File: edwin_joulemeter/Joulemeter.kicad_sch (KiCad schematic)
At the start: 17 parts, among them J1 Conn_01x02, J2 Conn_01x02, U1 INA240A3PWR, U2 ADS131M04IRUKR, U3 TLV709A01DBVR, U4 TPS7B92050DBVR

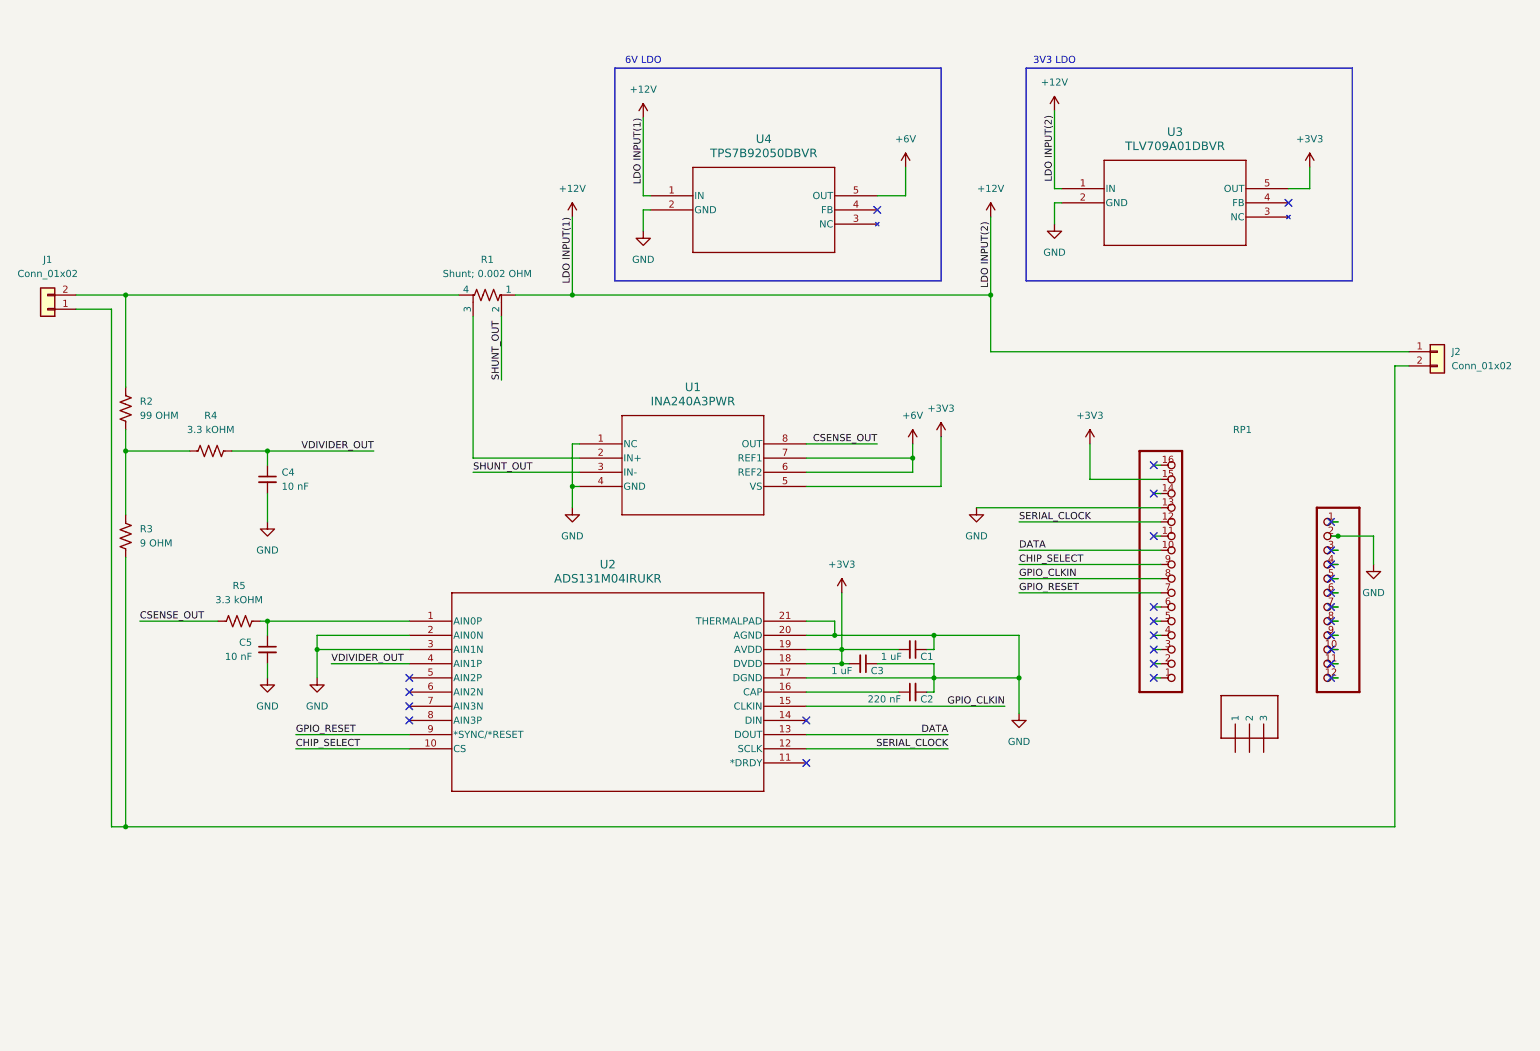
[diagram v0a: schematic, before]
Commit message: updated 1/5/25
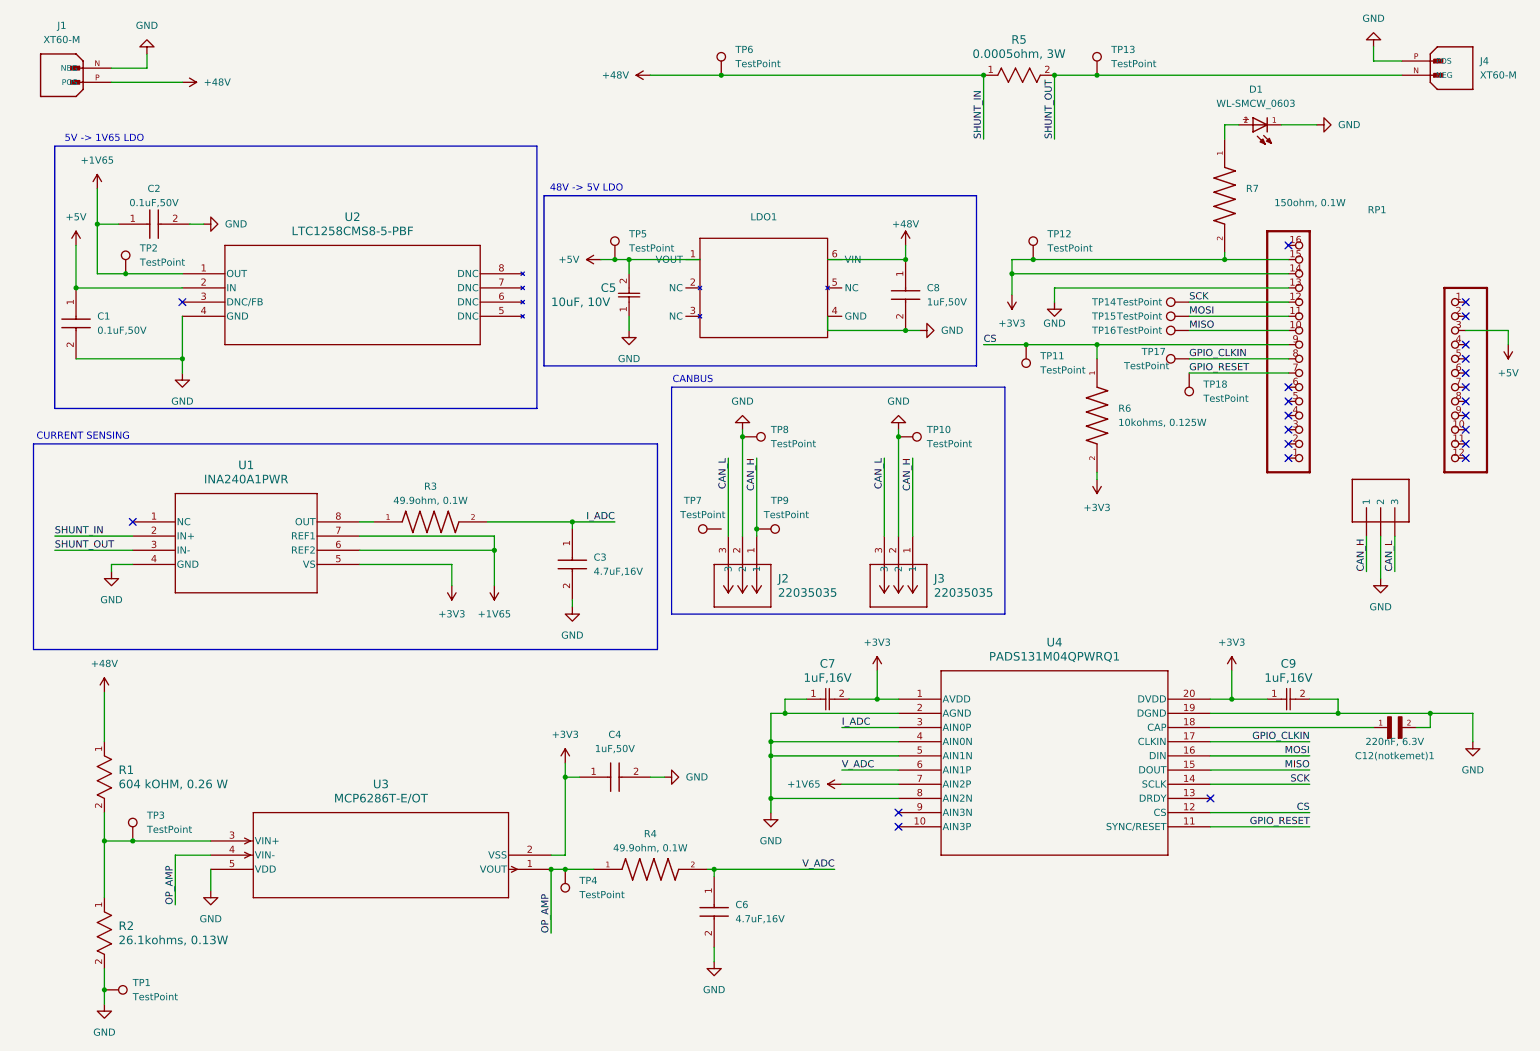
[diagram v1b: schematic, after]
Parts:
- removed C1, C3: 1 uF, symbol Device:C_Small
- removed C2: 220 nF, symbol Device:C_Small
- removed C4, C5: 10 nF, symbol Device:C_Small
- removed J1, J2: Conn_01x02, symbol Connector_Generic:Conn_01x02
- removed R1: Shunt; 0.002 OHM, symbol Device:R_Shunt_US
- removed R2: 99 OHM, symbol Device:R_US
- removed R3: 9 OHM, symbol Device:R_US
- removed R4, R5: 3.3 kOHM, symbol Device:R_US
- removed U2: ADS131M04IRUKR, RUK20_TEX, symbol Joulemeter:ADS131M04IRUKR
- removed U3: TLV709A01DBVR, SOT-23-5_DBV_TEX, symbol Joulemeter:TLV709A01DBVR
- removed U4: TPS7B92050DBVR, SOT-23-5_DBV_TEX, symbol Joulemeter:TLV709A01DBVR
- added C1, C2: 0.1uF,50V, C0805, symbol SMV_Custom:C0805C104K5RACTU
- added C12(notkemet)1: 220nF, 6.3V, SMV_Passives:0805RESC2012X60N, symbol SMV_Custom:GCM188R71H104KA57D
- added C3, C6: 4.7uF,16V, SMV_Passives:Cap0805, symbol SMV_Custom:C0805C475K4RACTU
- added C4, C8: 1uF,50V, C0805, symbol SMV_Custom:C0805C102K5GACTU
- added C5: 10uF, 10V, CAP_8PACTU, symbol SMV_Custom:C0805C106K8PACTU
- added C7, C9: 1uF,16V, SMV_Passives:Cap0805, symbol SMV_Custom:C0805C105K4RACTU
- added D1: WL-SMCW_0603, WL-SMCW_0603:WL-SMCW_0603, symbol SMV_Custom:WL-SMCW_0603
- added J1, J4: XT60-M, XT60-M:AMASS_XT60-M, symbol SMV_Custom:XT60-M
- added J2, J3: 22035035, CON_22035035_MOL, symbol SMV_Custom:3-pin Mini Molex Spox
- added LDO1: ~, symbol SMV_Custom:AP7387-50FDCR-7
- added R1: 604 kOHM, 0.26 W, RES_TNPW0805_VIS, symbol SMV_Custom:TNPW0805604KBEEA
- added R2: 26.1kohms, 0.13W, RES_TNPW0402_VIS, symbol SMV_Custom:TNPW040226K1BEED
- added R3, R4: 49.9ohm, 0.1W, CRCW060349R9FKEAC:RESC1608X55N, symbol SMV_Custom:CRCW060349R9FKEAC
- added R5: 0.0005ohm, 3W, RES_PU3921_.5mOHM_YAG, symbol SMV_Custom:PU3921FKM130U5L
- added R6: 10kohms, 0.125W, CRCW080510K0FKEAC:RESC2012X60N, symbol SMV_Custom:CRCW080510K0FKEAC
- added R7: 150ohm, 0.1W, CRCW0603150RFKEAC:RESC1608X55N, symbol SMV_Custom:CRCW0603150RFKEAC
- added TP1, TP10, TP11, TP12, TP13, TP14, TP15, TP16, TP17, TP18, TP2, TP3, TP4, TP5, TP6, TP7, TP8, TP9: TestPoint, TestPoint:TestPoint_Pad_3.0x3.0mm, symbol Connector:TestPoint
- added U2: LTC1258CMS8-5-PBF, MSOP-8_MS_LIT, symbol SMV_Custom:LTC1258CMS8-5-PBF
- added U3: MCP6286T-E/OT, SOT-23-5_MC_MCH, symbol SMV_Custom:MCP6286T-E_OT
- added U4: PADS131M04QPWRQ1, SMV_ICs:TSSOP20_PW_TEX, symbol SMV_Custom:PADS131M04QPWRQ1
- U1: value INA240A3PWR -> INA240A1PWR
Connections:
- net CHIP_SELECT is gone; now on net CS: RP1.9
- net DATA is gone; now on net MISO: RP1.10
- net SERIAL_CLOCK is gone; now on net SCK: RP1.12
- net +3V3: now also RP1.14, C4.1, C7.2, C9.1, R6.2, R7.2, TP12.1, U3.2 (VSS), U4.1 (AVDD), U4.20 (DVDD)
- net GND: now also C1.2, C12(notkemet)1.2, C2.2, C3.2, C4.2, C5.1, C6.2, C7.1, C8.2, C9.2, D1.1, J1.N (NEG), J2.2, J3.2, J4.P (POS), LDO1.4 (GND), R2.2, TP1.1, TP10.1, TP8.1, U2.4 (GND), U3.5 (VDD), U4.19 (DGND), U4.2 (AGND), U4.4 (AIN0N), U4.5 (AIN1N), U4.8 (AIN2N); no longer U1.1 (NC)
- net GPIO_CLKIN: now also TP17.1, U4.17 (CLKIN)
- net GPIO_RESET: now also TP18.1, U4.11 (SYNC/RESET)
- net SHUNT_OUT: now also J4.N (NEG), R5.2, TP13.1
- net +48V: now reaches U1.2 (IN+)
- net +48V: now also C8.1, J1.P (POS), LDO1.6 (VIN), R1.1, R5.1, TP6.1
- net CAN_H: now reaches RP1.1
- net CAN_H: now also J2.1, J3.1, TP9.1
- net MISO: now reaches RP1.10
- net MISO: now also TP16.1, U4.15 (DOUT)
- net MOSI: now reaches RP1.11
- net MOSI: now also TP15.1, U4.16 (DIN)
- net SCK: now reaches RP1.12
- net SCK: now also TP14.1, U4.14 (SCLK)
- net CAN_L: now reaches RP1.3
- net CAN_L: now also J2.3, J3.3
- net CS: now reaches RP1.9
- net CS: now also R6.1, TP11.1, U4.12 (CS)
- net +6V renamed +1V65
- net +1V65: now also C2.1, TP2.1, U2.1 (OUT), U4.7 (AIN2P)
- net CSENSE_OUT: no longer names the net of U1.8 (OUT)
- net CSENSE_OUT: now also R3.1
- new net: R1.2, R2.1, TP3.1, U3.3 (VIN+)
- new net: C12(notkemet)1.1, U4.18 (CAP)
- new net: D1.2, R7.1
- new net +5V: C1.1, C5.2, LDO1.1 (VOUT), RP1.3, TP5.1, U2.2 (IN)
- new net I_ADC: C3.1, R3.2, U4.3 (AIN0P)
- new net OP_AMP: R4.1, TP4.1, U3.1 (VOUT), U3.4 (VIN-)
- new net V_ADC: C6.1, R4.2, U4.6 (AIN1P)
- no-connect marks 28 -> 23
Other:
- note added: "48V -> 5V LDO"
- note added: "5V -> 1V65 LDO"
- note added: "CANBUS"
- note added: "CURRENT SENSING"
- note removed: "3V3 LDO"
- note removed: "6V LDO"

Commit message: updates to pcb/schematic for 1/7/2025
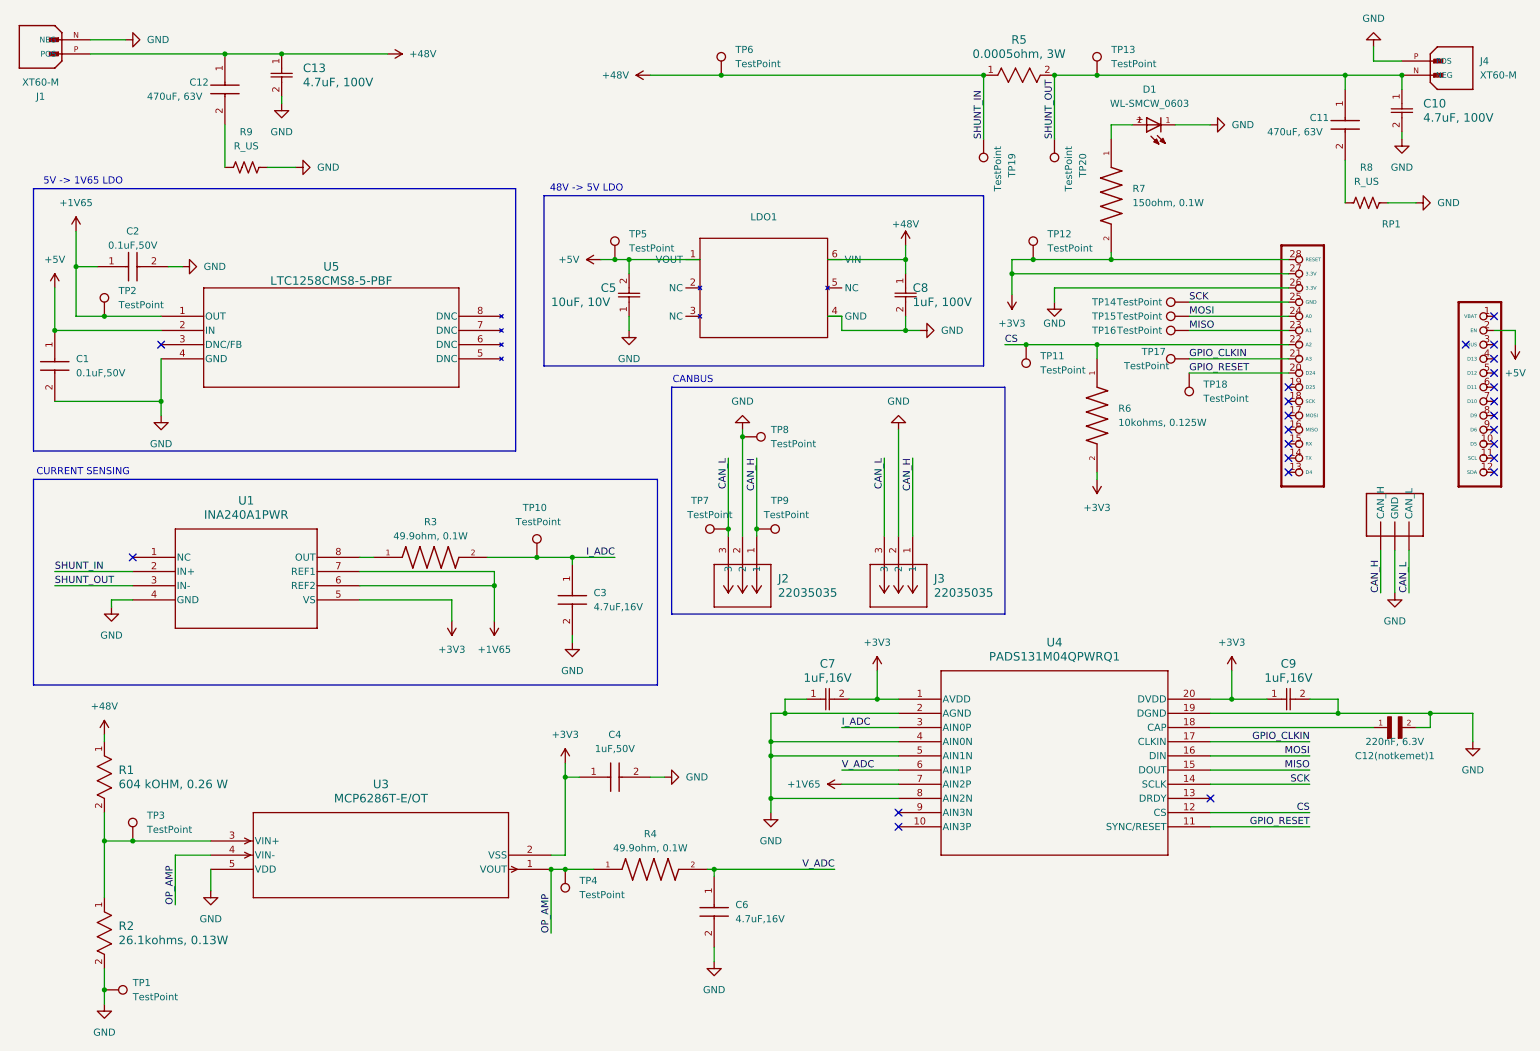
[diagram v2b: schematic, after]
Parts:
- removed C8: 1uF,50V, C0805, symbol SMV_Custom:C0805C102K5GACTU
- removed U2: LTC1258CMS8-5-PBF, MSOP-8_MS_LIT, symbol SMV_Custom:LTC1258CMS8-5-PBF
- added C10: 4.7uF, 100V, SMV_Passives:CAP_C2220C_2S_KEM, symbol SMV_Custom:C2220C475M1R2C7186
- added C11, C12: 470uF, 63V, SMV_Passives:Big_Chunky_Cap, symbol SMV_Custom:Big_Chunky_Cap2
- added C13: 4.7uF, 100V, CAP_C2220C_2S_KEM, symbol SMV_Custom:C2220C475M1R2C7186
- added C8: 1uF, 100V, SMV_Passives:CAPC340180_180N_KEM, symbol SMV_Custom:C1206C105K1RACTU
- added R8, R9: R_US, Resistor_THT:R_Axial_DIN0204_L3.6mm_D1.6mm_P1.90mm_Vertical, symbol Device:R_US
- added TP19, TP20: TestPoint, TestPoint:TestPoint_Pad_3.0x3.0mm, symbol Connector:TestPoint
- added U5: LTC1258CMS8-5-PBF, SMV_ICs:MSOP-8_MS_LIT, symbol SMV_Custom:LTC1258CMS8-5-PBF
- C1, C2, C4: footprint C0805 -> SMV_Passives:Cap0805
- C5: footprint CAP_8PACTU -> SMV_Passives:CAP_8PACTU
- D1: footprint WL-SMCW_0603:WL-SMCW_0603 -> SMV_Passives:WL-SMCW_0603(diode)
- J1, J4: footprint XT60-M:AMASS_XT60-M -> SMV_Connectors:AMASS_XT60-M
- J2, J3: footprint CON_22035035_MOL -> SMV_Connectors:3pin_CON_22035035_MOL
- LDO1: footprint (none) -> SMV_ICs:U-DFN2020-6 (Type C)
- R1: footprint RES_TNPW0805_VIS -> SMV_Passives:RES_TNPW0805_VIS
- R2: footprint RES_TNPW0402_VIS -> SMV_Passives:RES_TNPW0402_VIS
- R3, R4: footprint CRCW060349R9FKEAC:RESC1608X55N -> SMV_Passives:RESC1608X55N
- R5: footprint RES_PU3921_.5mOHM_YAG -> SMV_Passives:RES_PU3921_.5mOHM_YAG
- R6: footprint CRCW080510K0FKEAC:RESC2012X60N -> SMV_Passives:0805RESC2012X60N
- R7: footprint CRCW0603150RFKEAC:RESC1608X55N -> SMV_Passives:RESC1608X55N
- RP1: footprint (none) -> SMV_Connectors:RP2040
- U1: footprint PW0008A_N_TEX -> SMV_ICs:PW0008A_N_TEX
- U3: footprint SOT-23-5_MC_MCH -> SMV_ICs:SOT-23-5_MC_MCH
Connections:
- net +1V65: now also U5.1 (OUT)
- net +3V3: now also RP1.27 (3.3V), RP1.28 (RESET); no longer RP1.14, RP1.15
- net +48V: now also C12.1, C13.1, C8.1, TP19.1
- net +5V: now also RP1.2 (EN), U5.2 (IN); no longer RP1.3
- net CAN_H: now also RP1.31 (CAN_H); no longer RP1.1
- net CAN_L: now also RP1.29 (CAN_L), TP7.1; no longer RP1.3
- net CS: now also RP1.22 (A2); no longer RP1.9
- net GND: now also RP1.26 (3.3V), RP1.30 (GND), C10.2, C13.2, C8.2, R8.1, R9.1, U5.4 (GND); no longer RP1.13, RP1.2, TP10.1
- net GPIO_CLKIN: now also RP1.21 (A3); no longer RP1.8
- net GPIO_RESET: now also RP1.20 (D24); no longer RP1.7
- net I_ADC: now also TP10.1
- net MISO: now also RP1.23 (A1); no longer RP1.10
- net MOSI: now also RP1.24 (A0); no longer RP1.11
- net SCK: now also RP1.25 (GND); no longer RP1.12
- net SHUNT_OUT: now also C10.1, C11.1, TP20.1
- new net: C12.2, R9.2
- new net: C11.2, R8.2
- no-connect marks 23 -> 24
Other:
- moved on the sheet: C1, C2, C3, D1, J1, TP2, TP7, U1
